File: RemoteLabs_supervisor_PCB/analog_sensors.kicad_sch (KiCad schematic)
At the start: 12 parts, among them J22 Thermocouple A, U19 AD8497

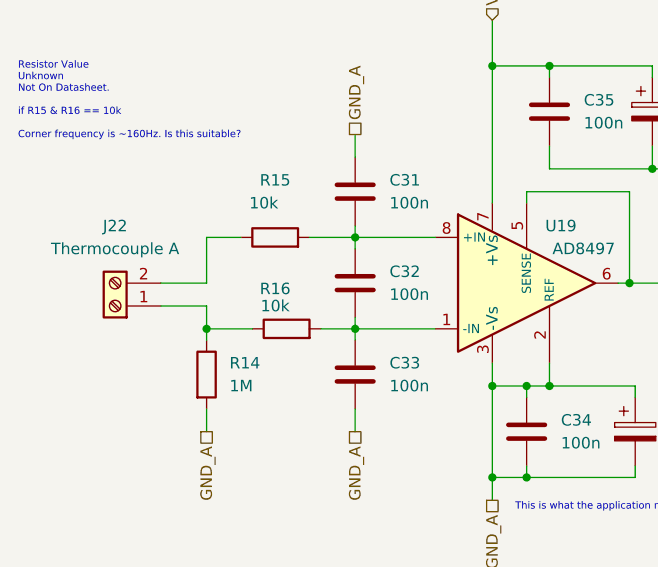
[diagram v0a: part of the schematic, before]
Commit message: mbncmvbc,
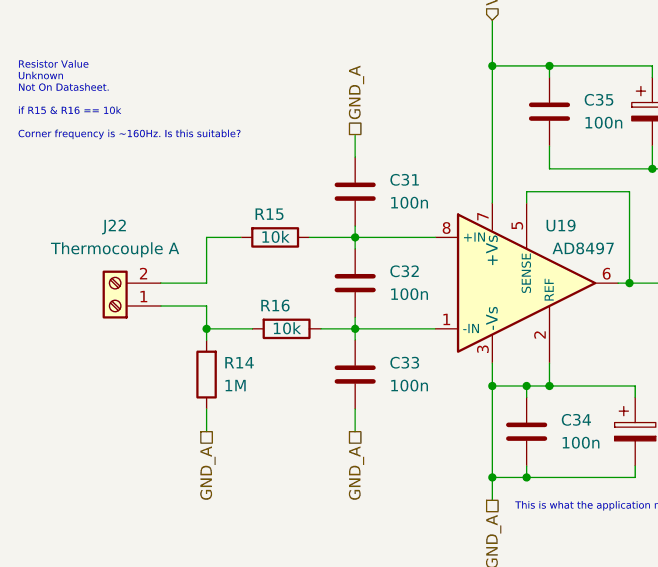
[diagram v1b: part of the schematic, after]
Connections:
- net GND_A: now also R14.1; no longer R14.2
- net at C31.2, C32.1, U19.8 (+IN): now also R15.1; no longer R15.2
- net at C32.2, C33.1, U19.1 (-IN): now also R16.1; no longer R16.2
- net at J22.2 (Pin_2): now also R15.2; no longer R15.1
- new net: J22.1 (Pin_1), R14.2, R16.2
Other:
- moved on the sheet: R14, R15, R16
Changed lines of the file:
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@@
     (pin "2")
   )
-  (symbol (lib_id "000_Resistors_Immo:Resistor_0805") (at 86.36 92.71 0) (unit 1)
-    (in_bom yes) (on_board yes) (fields_autoplaced)
-    (property "Reference" "R14" (id 0) (at 88.9 91.4399 0)
-      (effects (font (size 1.27 1.27)) (justify left))
+  (symbol (lib_id "000_Resistors_Immo:Resistor_0805") (at 86.36 92.71 90) (unit 1)
+    (in_bom yes) (on_board yes)
+    (property "Reference" "R14" (id 0) (at 88.265 91.44 90)
+      (effects (font (size 1.27 1.27)) (justify right))
     )
-    (property "Value" "1M" (id 1) (at 88.9 93.9799 0)
-      (effects (font (size 1.27 1.27)) (justify left))
+    (property "Value" "1M" (id 1) (at 88.265 93.98 90)
+      (effects (font (size 1.27 1.27)) (justify right))
     )
-    (property "Footprint" "Resistor_SMD:R_0805_2012Metric_Pad1.20x1.40mm_HandSolder" (id 2) (at 84.582 92.71 90)
+    (property "Footprint" "Resistor_SMD:R_0805_2012Metric_Pad1.20x1.40mm_HandSolder" (id 2) (at 86.36 94.488 90)
       (effects (font (size 1.27 1.27)) hide)
     )
@@
     (pin "2")
   )
-  (symbol (lib_id "000_Resistors_Immo:Resistor_0805") (at 95.25 87.63 90) (unit 1)
+  (symbol (lib_id "000_Resistors_Immo:Resistor_0805") (at 95.25 87.63 180) (unit 1)
     (in_bom yes) (on_board yes)
-    (property "Reference" "R16" (id 0) (at 93.98 83.185 90))
-    (property "Value" "10k" (id 1) (at 93.98 85.09 90))
-    (property "Footprint" "Resistor_SMD:R_0805_2012Metric_Pad1.20x1.40mm_HandSolder" (id 2) (at 95.25 89.408 90)
+    (property "Reference" "R16" (id 0) (at 93.98 85.09 0))
+    (property "Value" "10k" (id 1) (at 95.25 87.63 0))
+    (property "Footprint" "Resistor_SMD:R_0805_2012Metric_Pad1.20x1.40mm_HandSolder" (id 2) (at 97.028 87.63 90)
       (effects (font (size 1.27 1.27)) hide)
     )
@@
     (pin "2")
   )
-  (symbol (lib_id "000_Resistors_Immo:Resistor_0805") (at 93.98 77.47 90) (unit 1)
+  (symbol (lib_id "000_Resistors_Immo:Resistor_0805") (at 93.98 77.47 180) (unit 1)
     (in_bom yes) (on_board yes)
-    (property "Reference" "R15" (id 0) (at 93.98 71.12 90))
-    (property "Value" "10k" (id 1) (at 92.71 73.66 90))
-    (property "Footprint" "Resistor_SMD:R_0805_2012Metric_Pad1.20x1.40mm_HandSolder" (id 2) (at 93.98 79.248 90)
+    (property "Reference" "R15" (id 0) (at 93.345 74.93 0))
+    (property "Value" "10k" (id 1) (at 93.98 77.47 0))
+    (property "Footprint" "Resistor_SMD:R_0805_2012Metric_Pad1.20x1.40mm_HandSolder" (id 2) (at 95.758 77.47 90)
       (effects (font (size 1.27 1.27)) hide)
     )
